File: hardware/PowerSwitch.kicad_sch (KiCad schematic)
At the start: 2 parts, among them U701 TPS2559

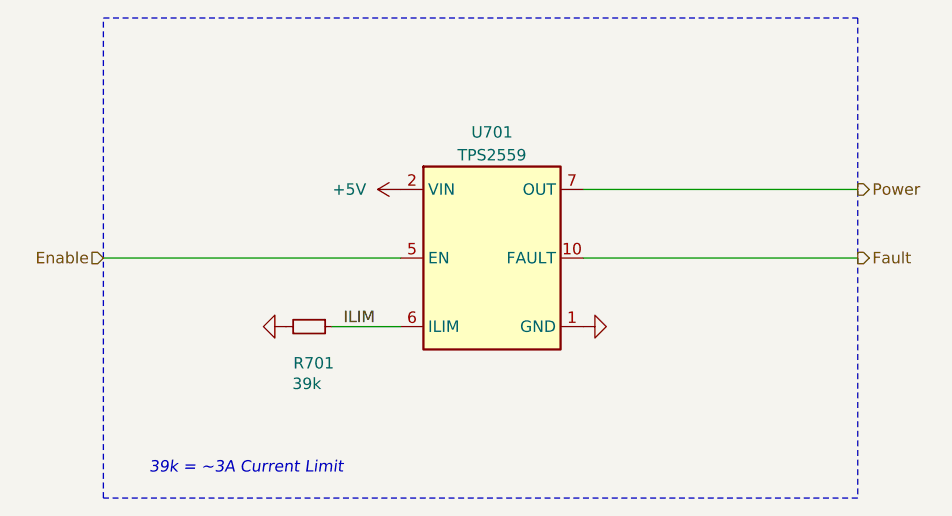
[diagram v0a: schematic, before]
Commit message: Refresh
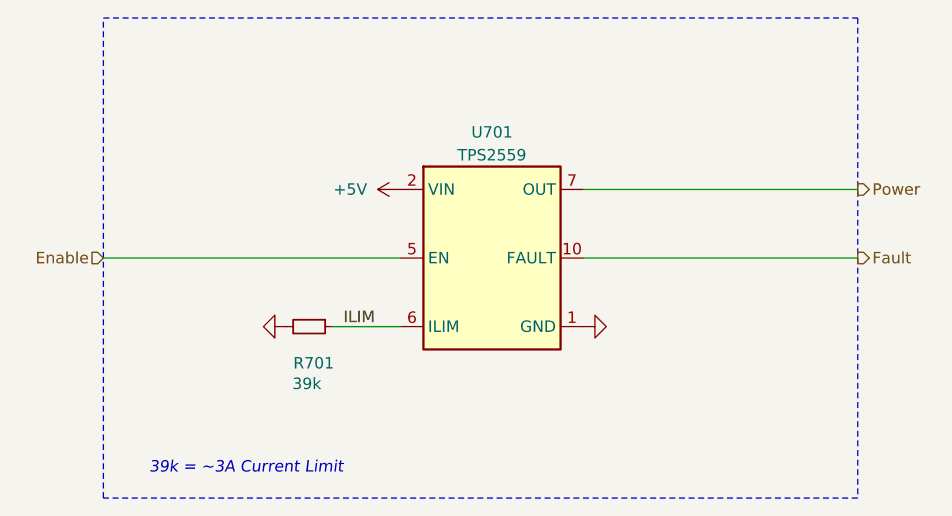
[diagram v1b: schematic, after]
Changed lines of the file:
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@@
 	(title_block
 		(title "V2 beat")
-		(date "2026-04-14")
-		(rev "2026-03-30")
+		(date "2026-08-11")
+		(rev "2026-08-11")
 		(company "Versio Duo")
 		(comment 1 "Solenoid Controller")
@@
 		(in_pos_files yes)
 		(dnp no)
-		(property "Reference" "#PWR0702"
+		(property "Reference" "#PWR702"
 			(at 149.86 99.06 0)
 			(hide yes)
@@
 		)
 		(property "Value" "+5V"
-			(at 142.24 99.06 90)
-			(show_name no)
-			(do_not_autoplace no)
-			(effects
-				(font
-					(size 1.27 1.27)
-				)
-				(justify left)
+			(at 140.462 99.06 90)
+			(show_name no)
+			(do_not_autoplace no)
+			(effects
+				(font
+					(size 1.27 1.27)
+					(color 255 92 187 1)
+				)
 			)
 		)
@@
 			(project "beat"
 				(path "/6c8448b4-b04d-47e1-934e-e40cbe27a7be/0ac9d349-3066-4d6a-93e7-4d57eaae463a"
-					(reference "#PWR0702")
+					(reference "#PWR702")
 					(unit 1)
 				)
@@
 		(dnp no)
 		(fields_autoplaced yes)
-		(property "Reference" "#PWR0701"
+		(property "Reference" "#PWR701"
 			(at 127 114.3 0)
 			(hide yes)
@@
 			(project "beat"
 				(path "/6c8448b4-b04d-47e1-934e-e40cbe27a7be/0ac9d349-3066-4d6a-93e7-4d57eaae463a"
-					(reference "#PWR0701")
+					(reference "#PWR701")
 					(unit 1)
 				)
@@
 			)
 		)
-		(property "Sim.Pin" ""
-			(at 156.21 106.68 0)
-			(hide yes)
-			(show_name no)
-			(do_not_autoplace no)
-			(effects
-				(font
-					(size 1.27 1.27)
-				)
-			)
-		)
-		(property "Voltage" ""
-			(at 156.21 106.68 0)
-			(hide yes)
-			(show_name no)
-			(do_not_autoplace no)
-			(effects
-				(font
-					(size 1.27 1.27)
-				)
-			)
-		)
 		(pin "1"
 		)
@@
 			)
 		)
-		(property "Sim.Pin" ""
-			(at 135.89 114.3 90)
-			(hide yes)
-			(show_name no)
-			(do_not_autoplace no)
-			(effects
-				(font
-					(size 1.27 1.27)
-				)
-			)
-		)
-		(property "Voltage" ""
-			(at 135.89 114.3 90)
-			(hide yes)
-			(show_name no)
-			(do_not_autoplace no)
-			(effects
-				(font
-					(size 1.27 1.27)
-				)
-			)
-		)
 		(pin "1"
 		)
@@
 		(dnp no)
 		(fields_autoplaced yes)
-		(property "Reference" "#PWR0703"
+		(property "Reference" "#PWR703"
 			(at 172.72 114.3 0)
 			(hide yes)
@@
 			(project "beat"
 				(path "/6c8448b4-b04d-47e1-934e-e40cbe27a7be/0ac9d349-3066-4d6a-93e7-4d57eaae463a"
-					(reference "#PWR0703")
+					(reference "#PWR703")
 					(unit 1)
 				)
